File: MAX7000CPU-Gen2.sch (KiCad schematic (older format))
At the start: 128 parts, among them J1 Conn_01x08_Male, J2 Conn_01x08_Male, J3 Conn_01x08_Male, J4 Conn_02x05_Odd_Even, J5 Conn_01x05_Male, SW1 SW_Push, SW2 SW_Push, SW3 SW_Push, U1 NE555P, U10 74LS241, U11 74LS241, U12 AS6C1008-55PCN, U13 74LS574, U14 74LS574, U15 CD4029BEE4, U16 CD4029BEE4, U17 CD4029BEE4, U18 CD4029BEE4, U19 74LS241, U2 NE555P, U20 74LS241, U21 74LS574, U22 74LS574, U23 74LS574, U24 74LS574, U25 74LS574, U26 74LS241, U27 74LS241, U28 EPM7128slc84-15n, U3 NE555P, U4 74LS574, U5 74LS574, U6 CD4029BEE4, U7 CD4029BEE4, U8 CD4029BEE4, U9 CD4029BEE4

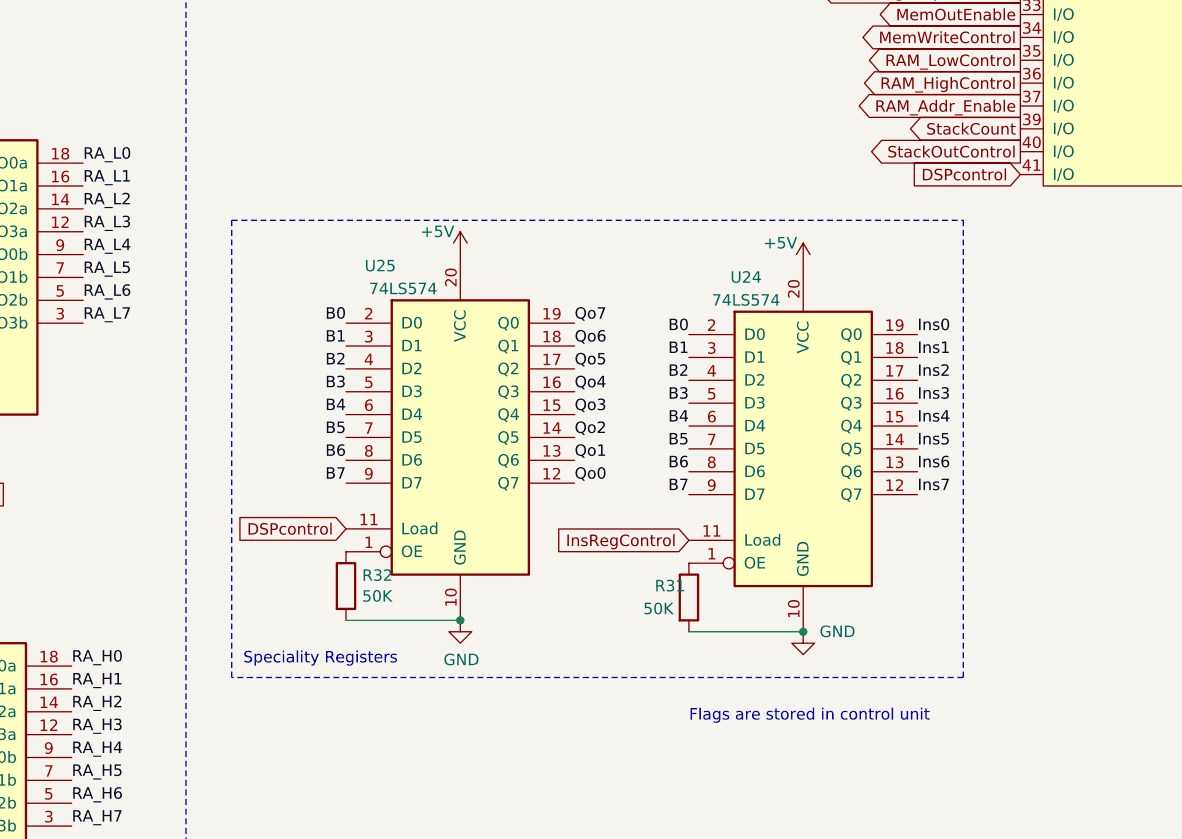
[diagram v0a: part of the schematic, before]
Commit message: controller timing
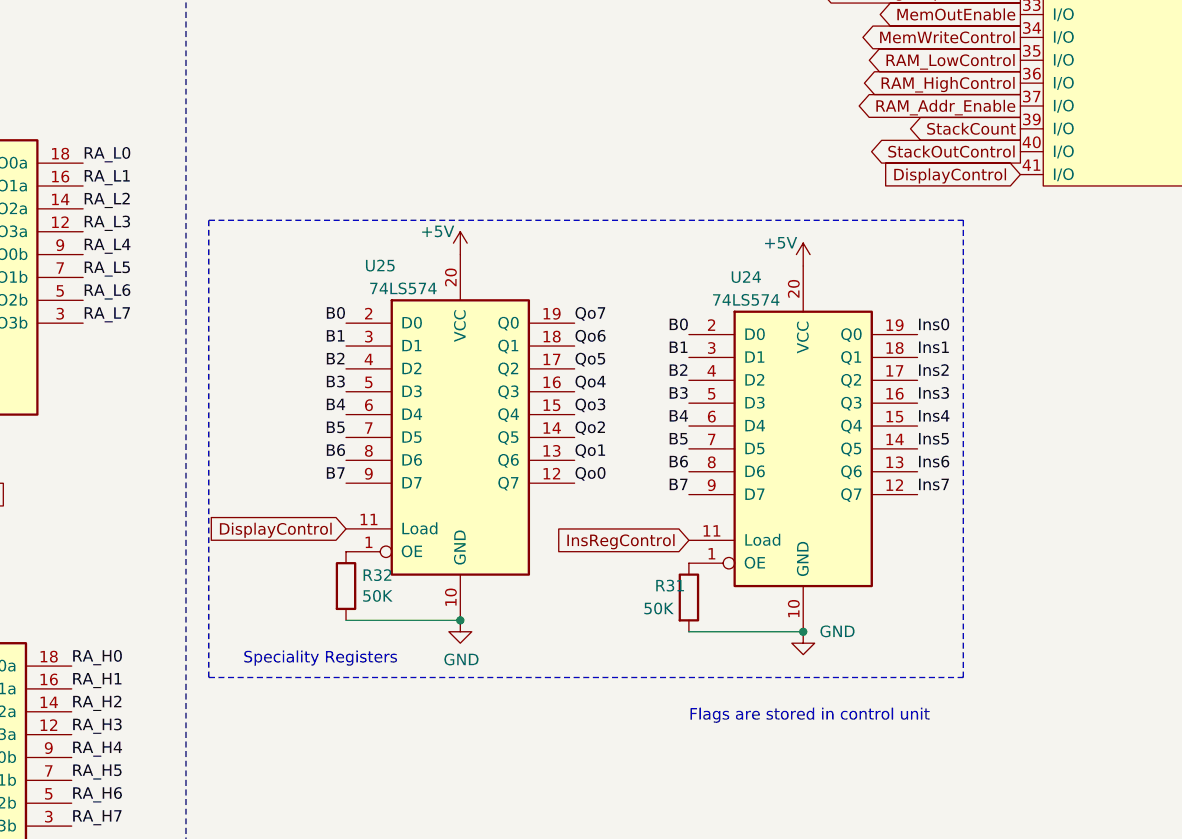
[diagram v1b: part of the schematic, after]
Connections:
- net DSPcontrol renamed DisplayControl
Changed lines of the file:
@@
 B7
 Text GLabel 10500 8800 0    50   Input ~ 0
-DSPcontrol
+DisplayControl
 Text Notes 10050 9400 0    50   ~ 0
 Speciality Registers
@@
 Flags are stored in control unit
 Text GLabel 13450 7250 0    50   Input ~ 0
-DSPcontrol
+DisplayControl
 Text GLabel 14550 7050 2    50   BiDi ~ 0
 CLK
@@
 	3800 4950 3800 5050
 Wire Notes Line
-	10000 7450 13200 7450
-Wire Notes Line
 	13200 7450 13200 9450
 Wire Notes Line
-	13200 9450 10000 9450
-Wire Notes Line
-	10000 7450 10000 9450
+	9900 7450 9900 9450
 Wire Wire Line
 	8250 10400 8250 10850
@@
 Wire Wire Line
 	10450 4150 12100 4150
+Wire Notes Line
+	9900 7450 13200 7450
+Wire Notes Line
+	9900 9450 13200 9450
 $EndSCHEMATC
